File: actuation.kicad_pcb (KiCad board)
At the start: 4 copper layers, 150 x 100 mm, 321 parts, among them J1 ACTUATION, J10 ACT CH9, J11 ACT CH10, J12 ACT CH11, J13 ACT CH12, J14 ACT CH13, J15 ACT CH14, J16 ACT CH15, J17 ACT CH16, J18 FB CH1, J19 FB CH2, J2 ACT CH1, J20 FB CH3, J21 VDET CH1, J22 VDET CH2, J23 PWR IN, J24 PWR PROT, J25 PWR 3.3V, J26 SAFETY, J27 ARM, J28 ACT HOT, J29 ACT COLD, J3 ACT CH2, J4 ACT CH3, J5 ACT CH4, J6 ACT CH5, J7 ACT CH6, J8 ACT CH7, J9 ACT CH8, K1 J115F11C, Q1 SI7220 NMOS, Q2 NMOS, U1 TPD4E02B04DQA, U10 TLP241A, U11 TLP241A, U12 TLP241A, U13 TLP241A, U14 TLP241A, U15 TLP241A, U16 TLP241A, U17 TLP241A, U18 TLP241A, U19 PCA9534, U2 PCA9615, U20 PCA9534, U21 TLP2366, U22 TLP2366, U23 TLP2366, U24 TLP2366, U25 TLP2366, U26 TLP2366, U27 TLV7031, U28 TLV7031, U29 TLP2366, U3 TLP241A, U30 TLP2366, U31 74LVC1G126, U32 74LVC1G126, U33 PCA9534, U34 SN74LVC541A, U35 TLI4971, U36 LTC4367, U37 ADS1110, U38 AP64350, U39 TLP241A, U4 TLP241A, U40 LP5912-3.3DRV, U5 TLP241A, U6 TLP241A, U7 TLP241A, U8 TLP241A, U9 TLP241A

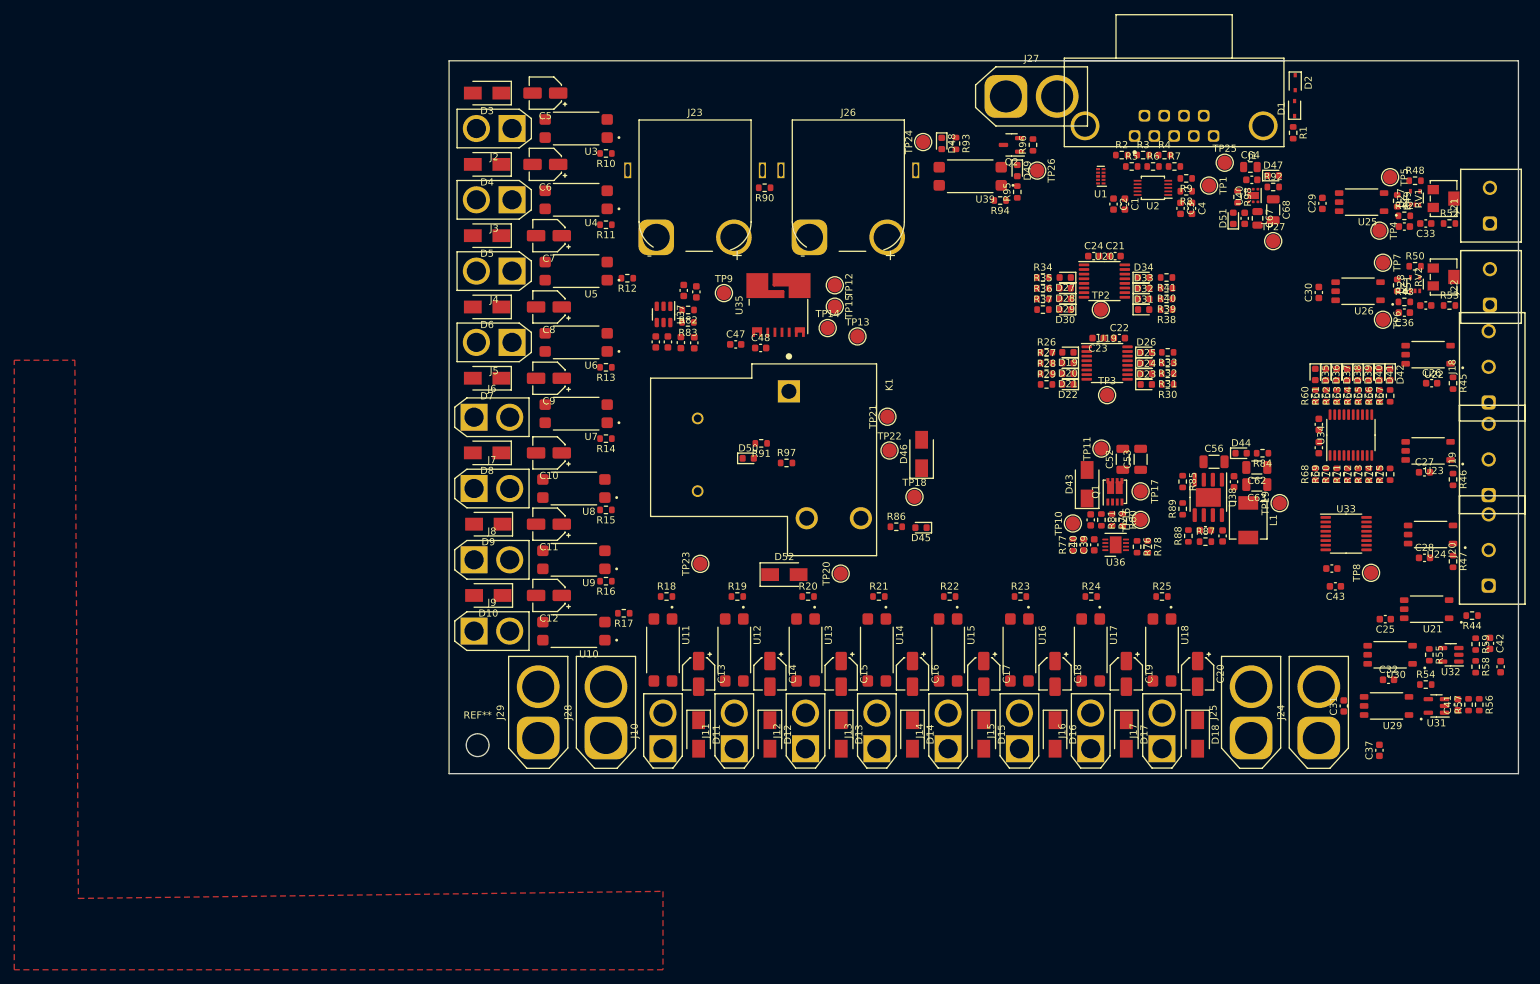
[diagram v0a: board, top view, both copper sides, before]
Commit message: 100x130
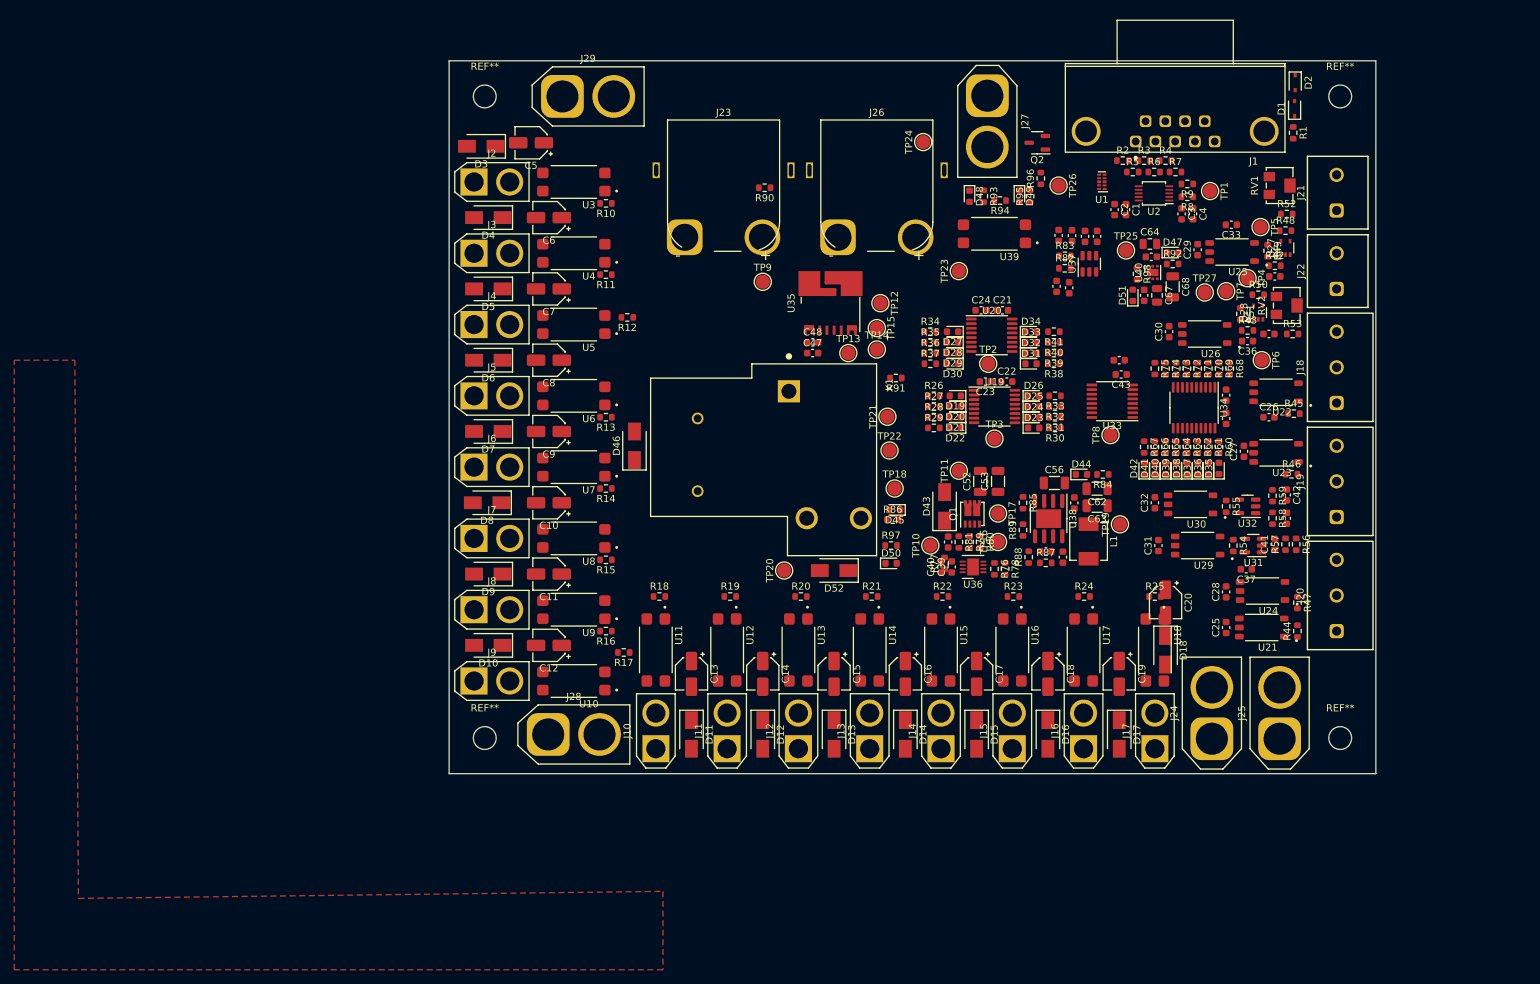
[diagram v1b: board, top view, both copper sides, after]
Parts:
- added REF**: MountingHole_3.2mm_M3, MountingHole:MountingHole_3.2mm_M3, F.Cu at (85.0, 45.0)
- added REF**: MountingHole_3.2mm_M3, MountingHole:MountingHole_3.2mm_M3, F.Cu at (205.0, 135.0)
- added REF**: MountingHole_3.2mm_M3, MountingHole:MountingHole_3.2mm_M3, F.Cu at (205.0, 45.0)
- moved J29 90.1 mm to (95.9, 45.0), turned to 0 degrees
- moved C57 63.7 mm to (170.9, 64.6), turned to 90 degrees
- moved C58 60.4 mm to (169.2, 64.6), turned to 90 degrees
- moved U37 60.1 mm to (169.8, 68.5), turned to 90 degrees
- moved C55 56.9 mm to (167.4, 64.5), turned to 90 degrees
- moved TP23 54.8 mm to (151.5, 69.5)
- moved C54 54.1 mm to (167.0, 71.8), turned to -90 degrees
- moved R83 53.7 mm to (166.4, 67.4), turned to 0 degrees
- moved C51 53.3 mm to (165.5, 64.5), turned to 90 degrees
- moved R82 53.2 mm to (166.4, 69.1), turned to 0 degrees
- moved C50 50.5 mm to (165.2, 71.6), turned to -90 degrees
- moved C43 42.3 mm to (174.3, 84.0)
- moved C45 41.8 mm to (174.0, 82.0)
- moved TP8 41.3 mm to (172.8, 92.5)
- moved C32 41.1 mm to (179.0, 102.0), turned to 90 degrees
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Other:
- board size 150 x 100 mm -> 130 x 100 mm
- board text added: "100 x 130 mm"

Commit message: Revert "100x130"
This reverts commit c49d85ffcdfed8898d048473301597551dfc5cab.
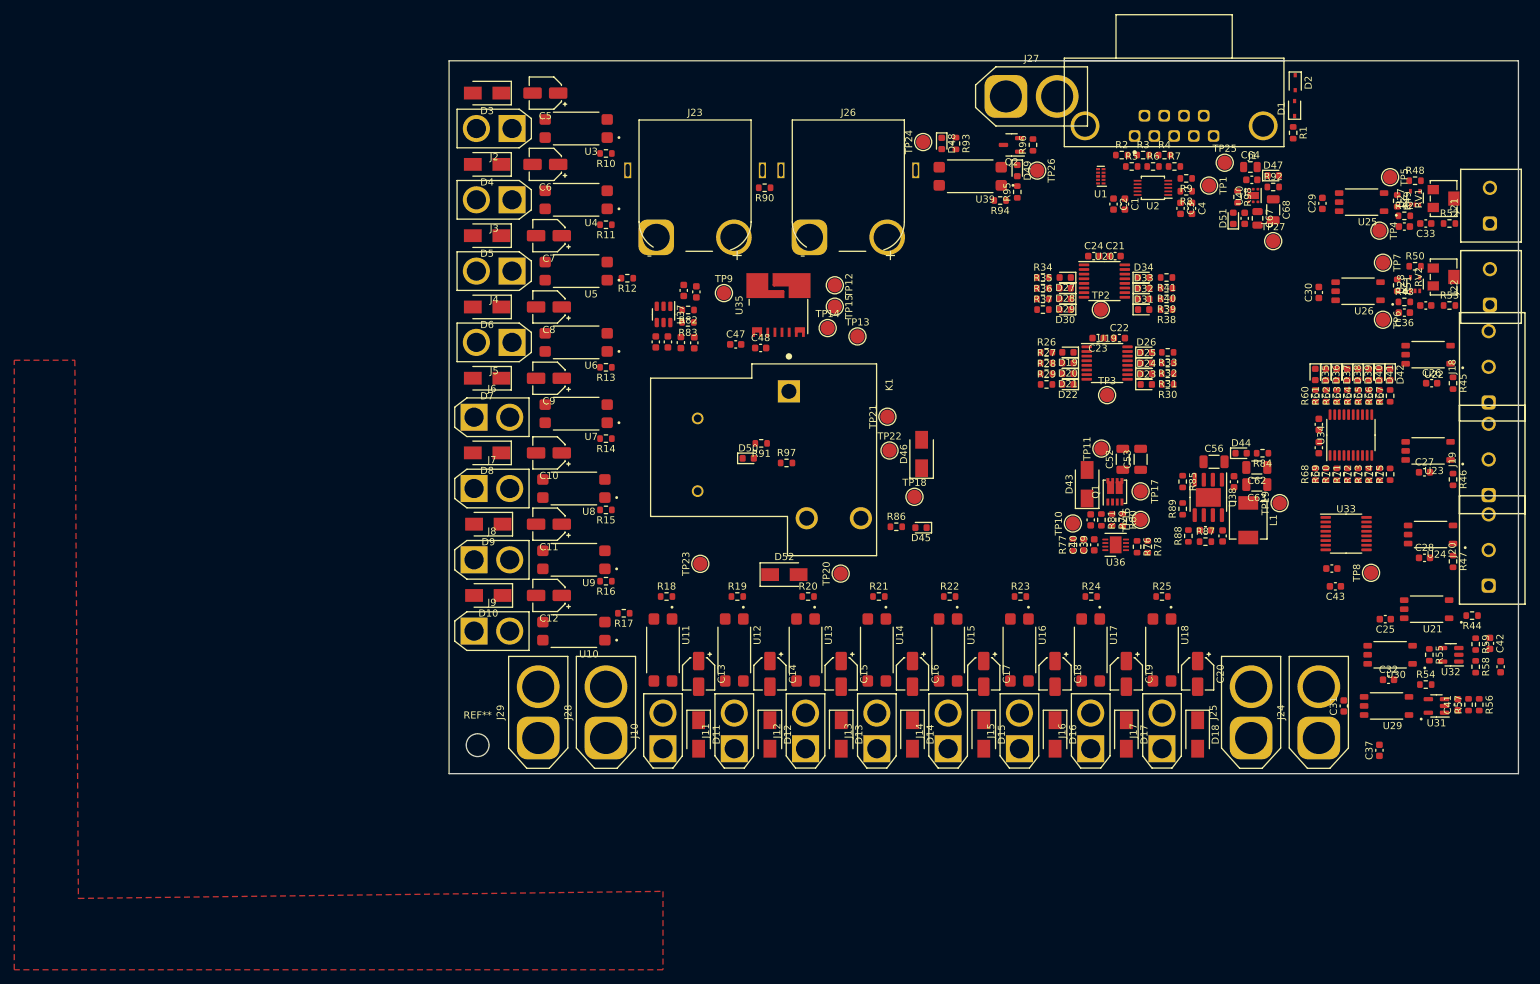
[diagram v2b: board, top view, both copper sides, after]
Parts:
- removed the REF** at (85.0, 45.0)
- removed the REF** at (205.0, 135.0)
- removed the REF** at (205.0, 45.0)
- moved J29 90.1 mm to (92.5, 135.0), turned to 90 degrees
- moved C57 63.7 mm to (109.0, 79.4), turned to -90 degrees
- moved C58 60.4 mm to (110.7, 79.4), turned to -90 degrees
- moved U37 60.1 mm to (110.1, 75.6), turned to -90 degrees
- moved C55 56.9 mm to (112.5, 79.5), turned to -90 degrees
- moved TP23 54.8 mm to (115.2, 110.6)
- moved C54 54.1 mm to (112.9, 72.2), turned to 90 degrees
- moved R83 53.7 mm to (113.5, 76.7), turned to 180 degrees
- moved C51 53.3 mm to (114.4, 79.6), turned to -90 degrees
- moved R82 53.2 mm to (113.5, 75.0), turned to 180 degrees
- moved C50 50.5 mm to (114.7, 72.4), turned to 90 degrees
- moved C43 42.3 mm to (204.3, 113.7)
- moved C45 41.8 mm to (203.8, 111.2)
- moved TP8 41.3 mm to (209.3, 111.8)
- moved C32 41.1 mm to (211.8, 126.8), turned to 0 degrees
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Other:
- board size 130 x 100 mm -> 150 x 100 mm
- board text removed: "100 x 130 mm"
